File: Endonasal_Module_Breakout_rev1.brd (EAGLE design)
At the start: 81.3 x 100 mm, 47 parts, among them J1 CONN_RECT_2X12TH, J2 CONN_RECT_2X12TH, J3 CONN_RECT_2X32NOHOLES, J4 CONN_RECT_2X20TH, J5 JACK_8P8C_RJ45_ETHERNET, J6 CONN_RECT_2X10TH, J7 CONN_RECT_2X10TH, U1 OR_M3, U2 OR_M0

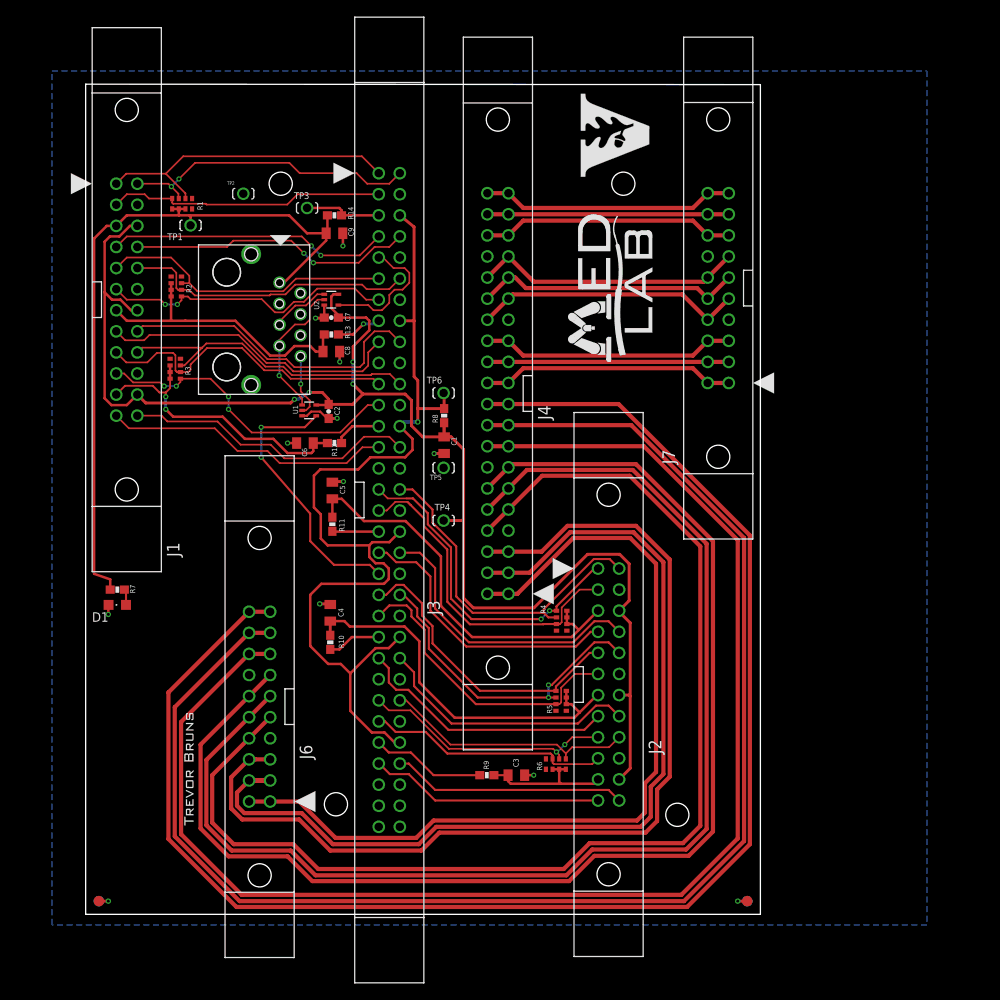
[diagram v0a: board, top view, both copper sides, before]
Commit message: Layout finished (hopefully)
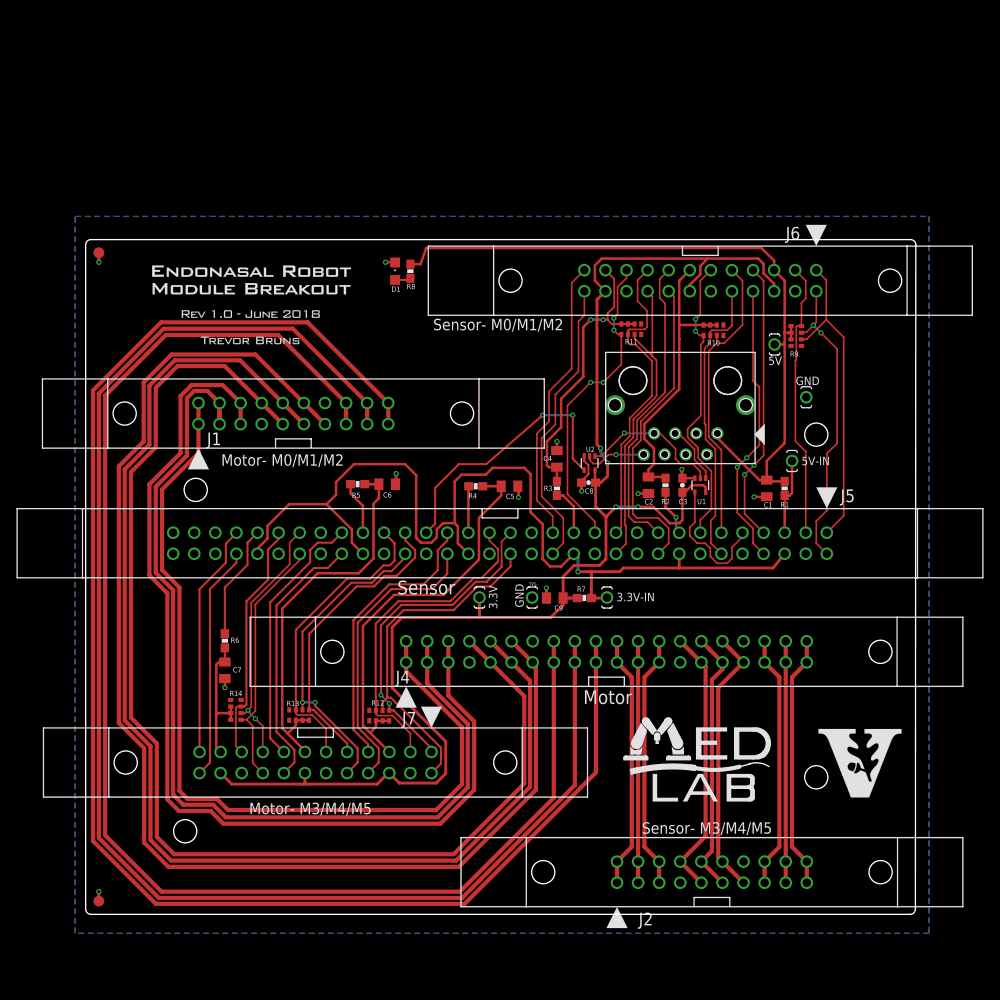
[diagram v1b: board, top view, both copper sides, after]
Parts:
- removed TP1, TP2, TP3, TP4, TP6: TEST-POINT_5021, Cannula_1_0:TEST-POINT_5021
- removed U$3: (no value), Cannula_1_0:LOGO_TREVOR_SMALL
- added 3.3V, 3.3V-IN, 5V, 5V-IN, GND: TEST-POINT_5021, Cannula_1_0:TEST-POINT_5021
- added U$5: (no value), Cannula_1_0:LOGO_ENDONASAL_BREAKOUT_1.0
- C2, C7: value 0.1uF -> 10uF; device SparkFun-Capacitors:0603-CAP -> Cannula_1_0:C0805K
- C3, C8: value 10uF -> 0.1uF; device Cannula_1_0:C0805K -> SparkFun-Capacitors:0603-CAP
- J1, J2: value CONN_RECT_2X12TH -> CONN_RECT_2X10TH; device Cannula_1_0:CONN_IDC_24_MALE_TH -> Cannula_1_0:CONN_IDC_20_MALE_TH
- J3: value CONN_RECT_2X32NOHOLES -> JACK_8P8C_RJ45_ETHERNET; device Cannula_1_0:CONN_IDC_64_MALE_TH_NOHOLES -> Cannula_1_0:ETHERNET_A104932
- J5: value JACK_8P8C_RJ45_ETHERNET -> CONN_RECT_2X32NOHOLES; device Cannula_1_0:ETHERNET_A104932 -> Cannula_1_0:CONN_IDC_64_MALE_TH_NOHOLES
- J6, J7: value CONN_RECT_2X10TH -> CONN_RECT_2X12TH; device Cannula_1_0:CONN_IDC_20_MALE_TH -> Cannula_1_0:CONN_IDC_24_MALE_TH
- R1, R2, R3, R4, R5, R6: value 10K -> 1; device SparkFun-Passives:0603-ARV -> Cannula_1_0:0603-RES
- R10, R11, R12, R13, R14, R9: value 1 -> 10K; device Cannula_1_0:0603-RES -> SparkFun-Passives:0603-ARV
- R7: value 220 -> 1
- R8: value 1 -> 220
- U1: value OR_M3 -> OR_M0
- U2: value OR_M0 -> OR_M3
- moved U$2 81.4 mm to (93.7, 18.9), turned to 0 degrees
- moved R1 80.3 mm to (84.2, 51.3), turned to 270 degrees
- moved TP10 78.1 mm to (1.59, 1.59), turned to 270 degrees
- moved TP7 78.1 mm to (1.59, 79.7), turned to 90 degrees
- moved TP8 78.1 mm to (1.59, 79.7), turned to 270 degrees
- moved TP9 78.1 mm to (1.59, 1.59), turned to 90 degrees
- moved J7 75.0 mm to (27.7, 18.3), turned to 180 degrees
- moved J6 73.8 mm to (74.0, 76.3), turned to 180 degrees
- moved R9 64.7 mm to (85.6, 69.7), turned to 270 degrees
- moved R2 63.6 mm to (69.8, 51.7), turned to 270 degrees
- moved R14 60.7 mm to (18.1, 24.6), turned to 90 degrees
- moved R10 59.5 mm to (75.6, 70.4), turned to 0 degrees
- moved U$4 58.8 mm to (74.1, 18.0), turned to 0 degrees
- moved R7 56.3 mm to (60.1, 38.1), turned to 0 degrees
- moved D1 52.3 mm to (37.3, 77.5), turned to 0 degrees
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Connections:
- net 3.3V: now also 3.3V.P$1, C3.1, C8.1, C9.1, J6.P$14, J6.P$22, J6.P$6, J7.P$14, J7.P$22, J7.P$6, R7.1; no longer C1.1, C2.1, C7.1, J1.P$14, J1.P$22, J1.P$6, J2.P$14, J2.P$22, J2.P$6, R8.1, TP4.P$1
- net 3.3V_IN: now also 3.3V-IN.P$1, J5.P$16, J5.P$26, J5.P$36, J5.P$46, J5.P$56, J5.P$6, R7.2; no longer J3.P$16, J3.P$26, J3.P$36, J3.P$46, J3.P$56, J3.P$6, R8.2, TP6.P$1
- net GND: now also GND.P$1, J3.SHIELD1, J3.SHIELD2, J5.P$10, J5.P$14, J5.P$20, J5.P$24, J5.P$30, J5.P$34, J5.P$4, J5.P$40, J5.P$44, J5.P$50, J5.P$54, J5.P$60, J6.P$12, J6.P$20, J6.P$4, J7.P$12, J7.P$20, J7.P$4; no longer J1.P$12, J1.P$20, J1.P$4, J2.P$12, J2.P$20, J2.P$4, J3.P$10, J3.P$14, J3.P$20, J3.P$24, J3.P$30, J3.P$34, J3.P$4, J3.P$40, J3.P$44, J3.P$50, J3.P$54, J3.P$60, J5.SHIELD1, J5.SHIELD2, TP2.P$1
- net LIMIT1: now also J3.P$5, U1.1; no longer J5.P$5, U2.1
- net LIMIT2: now also J3.P$7, U1.2, U2.1; no longer J5.P$7, U1.1, U2.2
- net LIMIT3: now also J3.P$8, U2.2; no longer J5.P$8, U1.2
- net M0A: now also J1.P$5, J1.P$6; no longer J6.P$5, J6.P$6
- net M0B: now also J1.P$3, J1.P$4; no longer J6.P$3, J6.P$4
- net M0C: now also J1.P$1, J1.P$2; no longer J6.P$1, J6.P$2
- net M0_ENC_A: now also J5.P$7, J6.P$7; no longer J1.P$7, J3.P$7
- net M0_ENC_B: now also J5.P$8, J6.P$8; no longer J1.P$8, J3.P$8
- net M0_HALL1: now also J5.P$1, J6.P$1, R9.6; no longer J1.P$1, J3.P$1, R1.6
- net M0_HALL2: now also J5.P$2, J6.P$2, R9.7; no longer J1.P$2, J3.P$2, R1.7
- net M0_HALL3: now also J5.P$3, J6.P$3, R9.8; no longer J1.P$3, J3.P$3, R1.8
- net M0_LIMIT: now also J5.P$9, U1.4; no longer J3.P$9, U2.4
- net M0_VHALL: now also 5V.P$1, C1.1, J3.P$1, J6.P$5, R8.2, R9.1, R9.2, R9.3; no longer C9.1, J1.P$5, J5.P$1, R1.2, R1.3, R14.1, R7.2, TP1.P$1
- net M0_VHALL_IN: now also 5V-IN.P$1, J5.P$5, R1.2; no longer J3.P$5, R14.2, TP3.P$1
- net M1A: now also J1.P$12, J1.P$13; no longer J6.P$12, J6.P$13
- net M1B: now also J1.P$10, J1.P$11; no longer J6.P$10, J6.P$11
- net M1C: now also J1.P$8, J1.P$9; no longer J6.P$8, J6.P$9
- net M1_ENC_A: now also J5.P$17, J6.P$15; no longer J1.P$15, J3.P$17
- net M1_ENC_B: now also J5.P$18, J6.P$16; no longer J1.P$16, J3.P$18
- net M1_HALL1: now also J5.P$11, J6.P$9, R10.3; no longer J1.P$9, J3.P$11, R2.3
- net M1_HALL2: now also J5.P$12, J6.P$10, R10.2; no longer J1.P$10, J3.P$12, R2.2
- net M1_HALL3: now also J5.P$13, J6.P$11, R10.1; no longer J1.P$11, J3.P$13, R2.1
- net M1_LIMIT: now also J5.P$19; no longer J3.P$19
- net M1_VHALL: now also C2.1, J6.P$13, R10.6, R10.7, R10.8, R2.1; no longer C8.1, J1.P$13, R13.1, R2.6, R2.7, R2.8
- net M1_VHALL_IN: now also J5.P$15, R2.2; no longer J3.P$15, R13.2
- net M2A: now also J1.P$19, J1.P$20; no longer J6.P$19, J6.P$20
- net M2B: now also J1.P$17, J1.P$18; no longer J6.P$17, J6.P$18
- net M2C: now also J1.P$15, J1.P$16; no longer J6.P$15, J6.P$16
- net M2_ENC_A: now also J5.P$27, J6.P$23; no longer J1.P$23, J3.P$27
- net M2_ENC_B: now also J5.P$28, J6.P$24; no longer J1.P$24, J3.P$28
- net M2_HALL1: now also J5.P$21, J6.P$17, R11.2; no longer J1.P$17, J3.P$21, R3.2
- net M2_HALL2: now also J5.P$22, J6.P$18, R11.3; no longer J1.P$18, J3.P$22, R3.3
- net M2_HALL3: now also J5.P$23, J6.P$19, R11.1; no longer J1.P$19, J3.P$23, R3.1
- net M2_LIMIT: now also J5.P$29; no longer J3.P$29
- net M2_VHALL: now also C4.1, J6.P$21, R11.6, R11.7, R11.8, R3.1; no longer C6.1, J1.P$21, R12.1, R3.6, R3.7, R3.8
- net M2_VHALL_IN: now also J5.P$25, R3.2; no longer J3.P$25, R12.2
- net M3A: now also J2.P$5, J2.P$6; no longer J7.P$5, J7.P$6
- net M3B: now also J2.P$3, J2.P$4; no longer J7.P$3, J7.P$4
- net M3C: now also J2.P$1, J2.P$2; no longer J7.P$1, J7.P$2
- net M3_ENC_A: now also J5.P$37, J7.P$7; no longer J2.P$7, J3.P$37
- net M3_ENC_B: now also J5.P$38, J7.P$8; no longer J2.P$8, J3.P$38
- net M3_HALL1: now also J5.P$31, J7.P$1, R12.1; no longer J2.P$1, J3.P$31, R4.1
- net M3_HALL2: now also J5.P$32, J7.P$2, R12.2; no longer J2.P$2, J3.P$32, R4.2
- net M3_HALL3: now also J5.P$33, J7.P$3, R12.3; no longer J2.P$3, J3.P$33, R4.3
- net M3_LIMIT: now also J5.P$39, U2.4; no longer J3.P$39, U1.4
- net M3_VHALL: now also J7.P$5, R12.6, R12.7, R12.8, R4.1; no longer J2.P$5, R11.1, R4.6, R4.7, R4.8
- net M3_VHALL_IN: now also J5.P$35, R4.2; no longer J3.P$35, R11.2
- net M4A: now also J2.P$12, J2.P$13; no longer J7.P$12, J7.P$13
- net M4B: now also J2.P$10, J2.P$11; no longer J7.P$10, J7.P$11
- net M4C: now also J2.P$8, J2.P$9; no longer J7.P$8, J7.P$9
- net M4_ENC_A: now also J5.P$47, J7.P$15; no longer J2.P$15, J3.P$47
- net M4_ENC_B: now also J5.P$48, J7.P$16; no longer J2.P$16, J3.P$48
- net M4_HALL1: now also J5.P$41, J7.P$9, R13.1; no longer J2.P$9, J3.P$41, R5.1
- net M4_HALL2: now also J5.P$42, J7.P$10, R13.2; no longer J2.P$10, J3.P$42, R5.2
- net M4_HALL3: now also J5.P$43, J7.P$11, R13.3; no longer J2.P$11, J3.P$43, R5.3
- net M4_LIMIT: now also J5.P$49; no longer J3.P$49
- net M4_VHALL: now also C6.1, J7.P$13, R13.6, R13.7, R13.8, R5.1; no longer C4.1, J2.P$13, R10.1, R5.6, R5.7, R5.8
- net M4_VHALL_IN: now also J5.P$45, R5.2; no longer J3.P$45, R10.2
- net M5A: now also J2.P$19, J2.P$20; no longer J7.P$19, J7.P$20
- net M5B: now also J2.P$17, J2.P$18; no longer J7.P$17, J7.P$18
- net M5C: now also J2.P$15, J2.P$16; no longer J7.P$15, J7.P$16
- net M5_ENC_A: now also J5.P$57, J7.P$23; no longer J2.P$23, J3.P$57
- net M5_ENC_B: now also J5.P$58, J7.P$24; no longer J2.P$24, J3.P$58
- net M5_HALL1: now also J5.P$51, J7.P$17, R14.2; no longer J2.P$17, J3.P$51, R6.2
- net M5_HALL2: now also J5.P$52, J7.P$18, R14.1; no longer J2.P$18, J3.P$52, R6.1
- net M5_HALL3: now also J5.P$53, J7.P$19, R14.3; no longer J2.P$19, J3.P$53, R6.3
- net M5_LIMIT: now also J5.P$59; no longer J3.P$59
- net M5_VHALL: now also C7.1, J7.P$21, R14.6, R14.7, R14.8, R6.1; no longer C3.1, J2.P$21, R6.6, R6.7, R6.8, R9.1
- net M5_VHALL_IN: now also J5.P$55, R6.2; no longer J3.P$55, R9.2
- net N$190: now also J5.P$62; no longer J3.P$62
- net N$191: now also J5.P$63; no longer J3.P$63
- net N$192: now also J5.P$64; no longer J3.P$64
- net N$6: now also R8.1; no longer R7.1
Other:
- board size 81.3 x 100 mm -> 100 x 81.3 mm
- board text added: "GND"
- board text added: "Motor"
- board text added: "Motor- M0/M1/M2"
- board text added: "Motor- M3/M4/M5"
- board text added: "Sensor"
- board text added: "Sensor- M0/M1/M2"
- board text added: "Sensor- M3/M4/M5"
